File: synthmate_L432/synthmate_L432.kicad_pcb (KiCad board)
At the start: 2 copper layers, 5 parts, among them U1 STM32L432KCUx, U3 MIC5365-1.0YC5

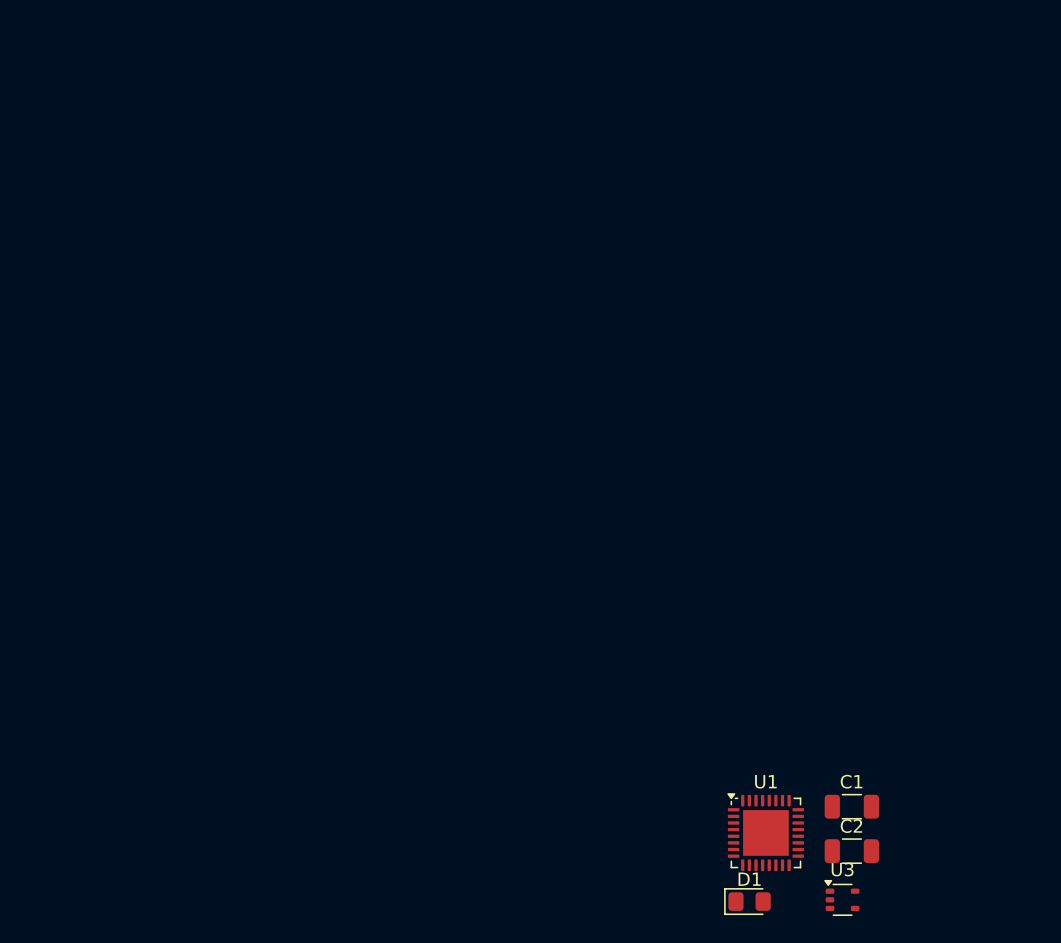
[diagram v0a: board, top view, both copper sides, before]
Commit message: pcb_v1
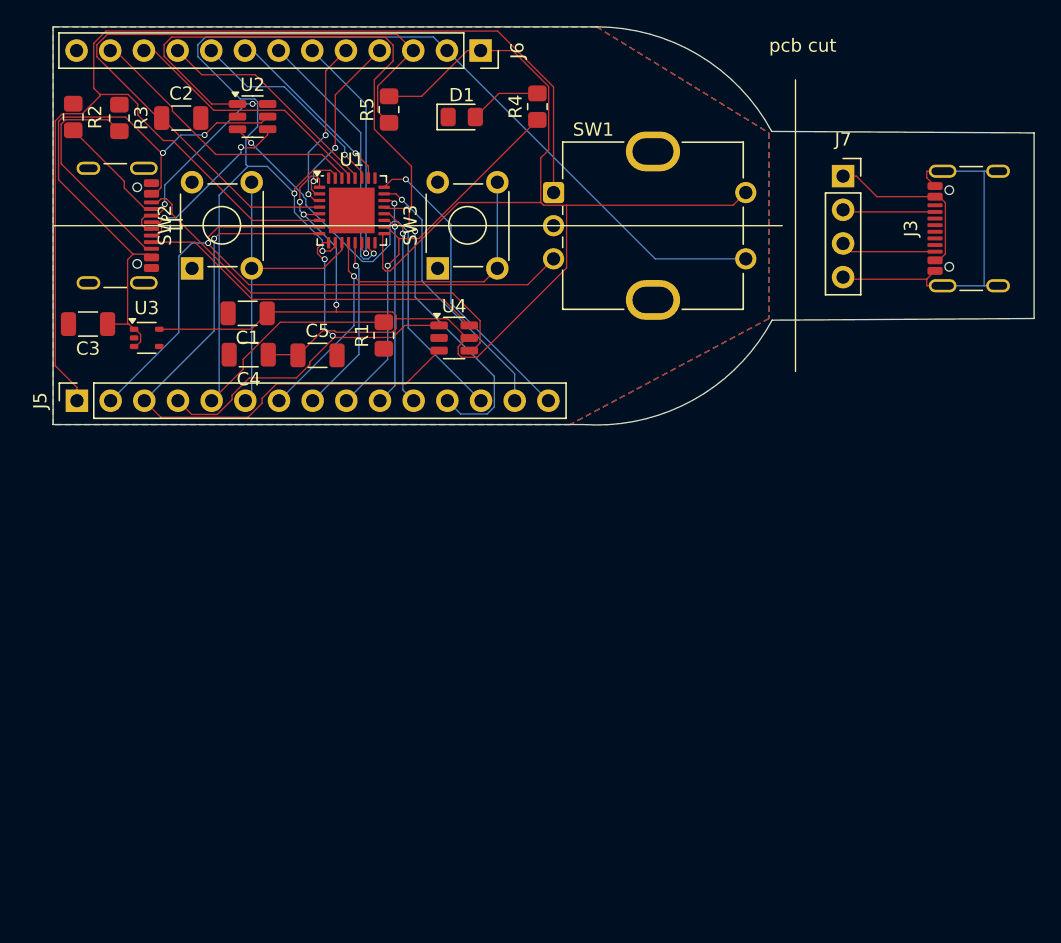
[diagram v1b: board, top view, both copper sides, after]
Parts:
- added C3: 1uF, Capacitor_SMD:C_1206_3216Metric, F.Cu at (93.6, 54.4)
- added C4: 1uF, Capacitor_SMD:C_1206_3216Metric, F.Cu at (105.8, 56.7)
- added C5: 100nF, Capacitor_SMD:C_1206_3216Metric, F.Cu at (110.9, 56.8)
- added J1: USB_C_synthmate, Connector_USB:USB_C_Receptacle_GCT_USB4105-xx-A_16P_TopMnt_Horizontal, F.Cu at (94.7, 47.0)
- added J3: USB_C_connector_board, Connector_USB:USB_C_Receptacle_GCT_USB4105-xx-A_16P_TopMnt_Horizontal, F.Cu at (161.2, 47.2)
- added J5: Conn_01x16, Connector_PinSocket_2.54mm:PinSocket_1x15_P2.54mm_Vertical, F.Cu at (92.8, 60.2)
- added J6: Conn_01x13, Connector_PinSocket_2.54mm:PinSocket_1x13_P2.54mm_Vertical, F.Cu at (123.2, 33.8)
- added J7: Conn_01x04, Connector_PinSocket_2.54mm:PinSocket_1x04_P2.54mm_Vertical, F.Cu at (150.6, 43.3)
- added R1: 10k, Resistor_SMD:R_0805_2012Metric_Pad1.20x1.40mm_HandSolder, F.Cu at (116.0, 55.3)
- added R2: 5k1, Resistor_SMD:R_0805_2012Metric_Pad1.20x1.40mm_HandSolder, F.Cu at (92.5, 38.8)
- added R3: 5k1, Resistor_SMD:R_0805_2012Metric_Pad1.20x1.40mm_HandSolder, F.Cu at (96.0, 38.9)
- added R4: 1k, Resistor_SMD:R_0805_2012Metric_Pad1.20x1.40mm_HandSolder, F.Cu at (127.5, 38.0)
- added R5: 10k, Resistor_SMD:R_0805_2012Metric_Pad1.20x1.40mm_HandSolder, F.Cu at (116.3, 38.2)
- added SW1: RotaryEncoder_Switch, Rotary_Encoder:RotaryEncoder_Bourns_Vertical_PEC12R-3x17F-Sxxxx, F.Cu at (128.8, 44.5)
- added SW2: SW_Push, Button_Switch_THT:SW_TH_Tactile_Omron_B3F-10xx, F.Cu at (101.5, 50.2)
- added SW3: SW_Push, Button_Switch_THT:SW_TH_Tactile_Omron_B3F-10xx, F.Cu at (120.0, 50.2)
- added U2: USBLC6-2SC6, Package_TO_SOT_SMD:SOT-23-6, F.Cu at (106.0, 38.8)
- added U4: USBLC6-2SC6, Package_TO_SOT_SMD:SOT-23-6, F.Cu at (121.3, 55.5)
- C1: value 16V/47uF Tantalum -> 16V/47uF
- moved C2 74.9 mm to (100.7, 38.9)
- moved U3 67.5 mm to (98.1, 55.5)
- moved D1 63.0 mm to (121.8, 38.8)
- moved C1 58.8 mm to (105.7, 53.6), turned to 180 degrees
- moved U1 56.4 mm to (113.5, 45.9)
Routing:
- net 3V3: track 0.00 -> 124.1 mm, vias 0 -> 3
- net BOOT0: track 0.00 -> 110.6 mm, vias 0 -> 2
- net enc_A: track 0.00 -> 95.9 mm
- net USB_DM: track 0.00 -> 63.5 mm, vias 0 -> 1
- net NRST: track 0.00 -> 54.0 mm
- net enc_B: track 0.00 -> 53.0 mm, vias 0 -> 1
- net LPUART_TX: track 0.00 -> 47.6 mm, vias 0 -> 1
- net 5V: track 0.00 -> 45.0 mm, vias 0 -> 2
- net USB_DP: track 0.00 -> 37.0 mm, vias 0 -> 2
- net pushbutton_B: track 0.00 -> 32.3 mm, vias 0 -> 1
- net Net-(J1-SBU2): track 0.00 -> 31.9 mm
- net LPUART_RX: track 0.00 -> 31.5 mm, vias 0 -> 2
- net LED: track 0.00 -> 29.5 mm, vias 0 -> 1
- net adaptor_GND: track 0.00 -> 28.5 mm
- net Net-(J1-SBU1): track 0.00 -> 26.6 mm
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- added copper zone on B.Cu, net GND
- added copper zone on F.Cu, net GND
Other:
- board outline added: 74 x 30 mm
- board text added: "pcb cut"
